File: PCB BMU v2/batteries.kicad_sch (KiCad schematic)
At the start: 19 parts, among them Q8 IRFZ44NPBF, U7 INA237

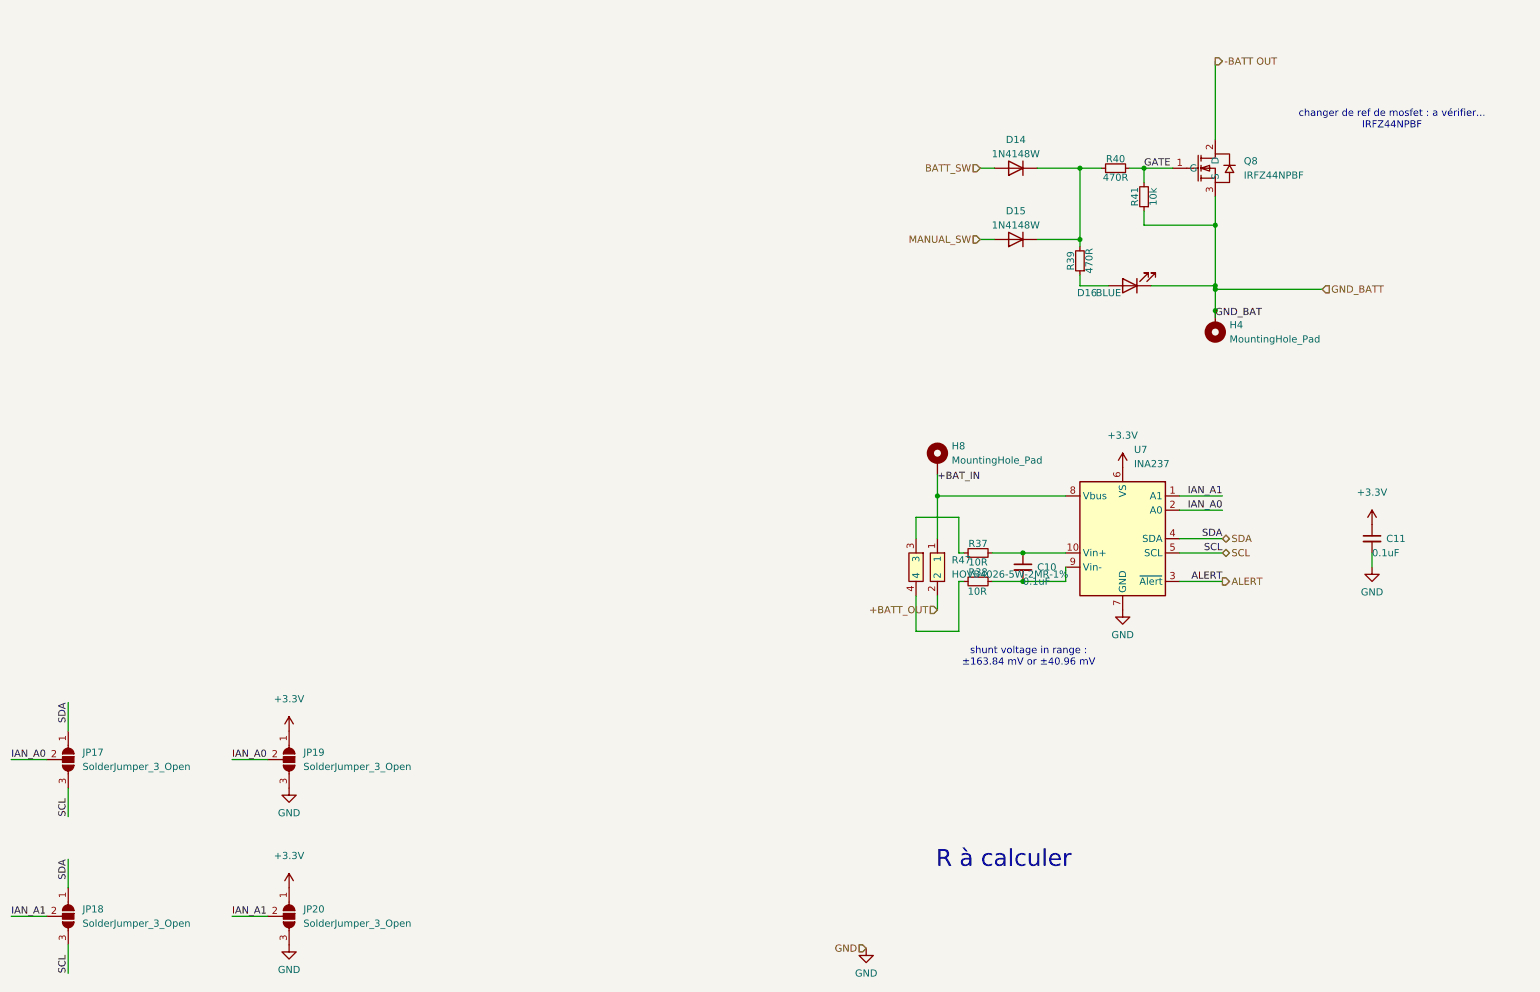
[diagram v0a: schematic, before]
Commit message: update code
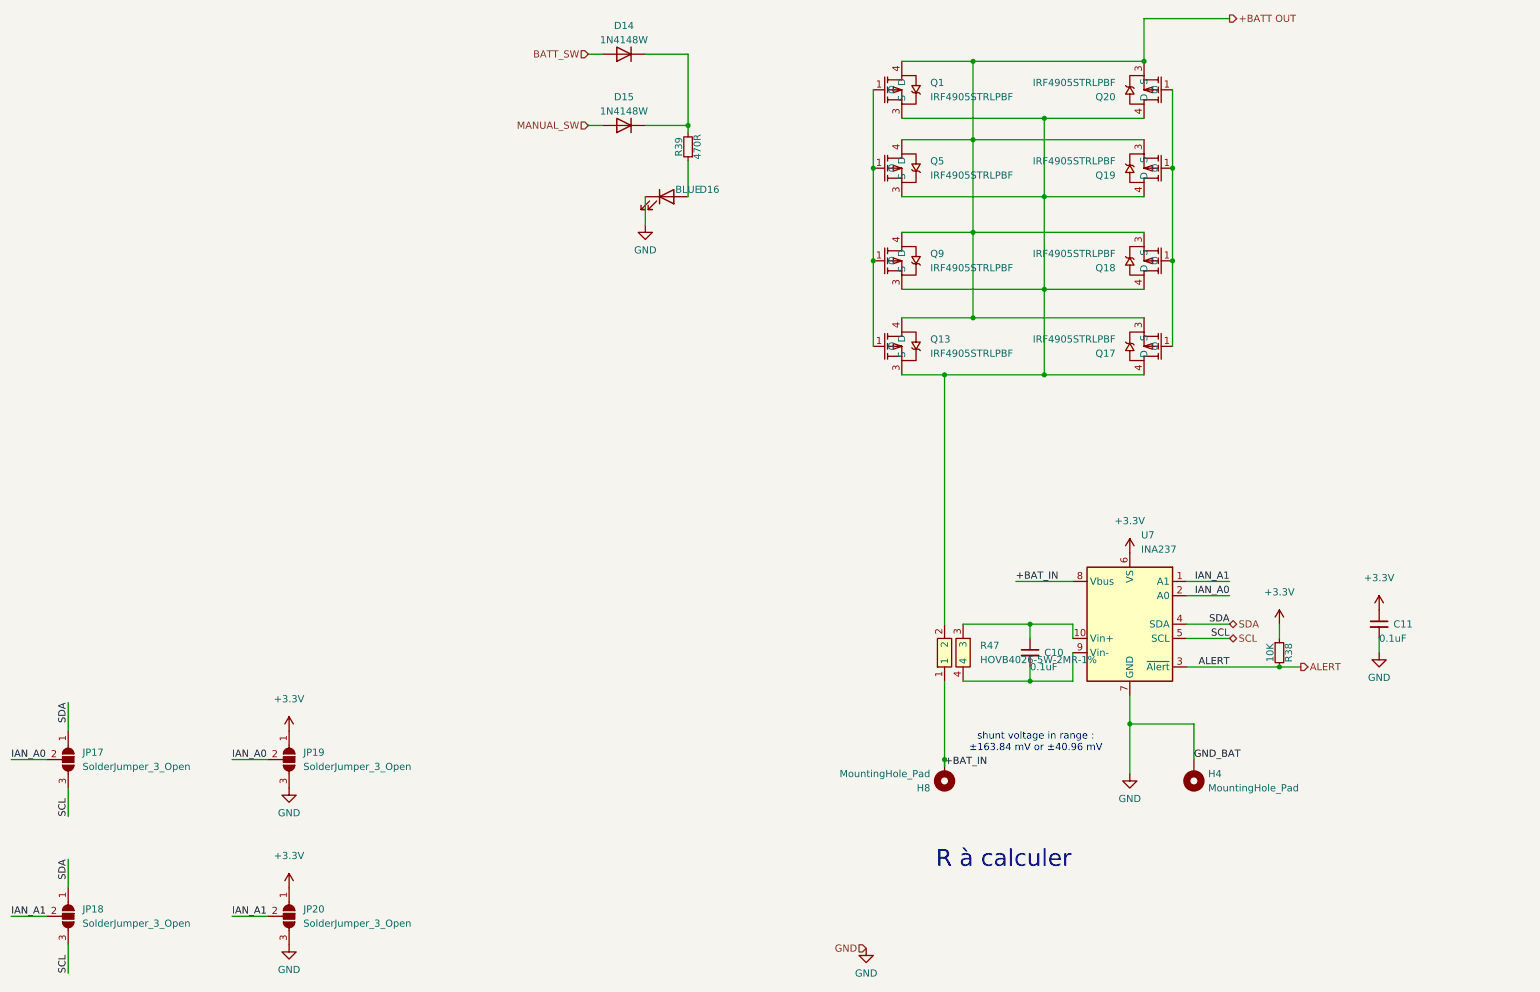
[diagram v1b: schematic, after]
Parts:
- removed Q8: IRFZ44NPBF, Package_TO_SOT_THT:TO-220-3_Horizontal_TabUp, symbol easyeda2kicad:IRFZ44NPBF
- removed R37: 10R, Resistor_SMD:R_0603_1608Metric, symbol Device:R_Small
- removed R40: 470R, Resistor_THT:R_Axial_DIN0204_L3.6mm_D1.6mm_P5.08mm_Horizontal, symbol Device:R_Small
- removed R41: 10k, Resistor_THT:R_Axial_DIN0204_L3.6mm_D1.6mm_P5.08mm_Horizontal, symbol Device:R_Small
- added Q1, Q13, Q17, Q18, Q19, Q20, Q5, Q9: IRF4905STRLPBF, easyeda2kicad:D2PAK_L9.1-W10.0-P2.54-LS15.3-TL, symbol easyeda2kicad:IRF4905STRLPBF
- C11: footprint Capacitor_SMD:C_0805_2012Metric -> Capacitor_SMD:C_0402_1005Metric; LCSC (none) -> C1525; LCSC Alt (none) -> C307331
- R38: value 10R -> 10K
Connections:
- net GND_BATT is gone; now on net GND: D16.1 (K), H4.1
- net +3.3V: now also R38.1
- net ALERT: now also R38.2
- net at R47.3: now also C10.1, U7.10 (Vin+)
- net at C10.2, U7.9 (Vin-): now also R47.4; no longer R38.1
- net +BATT_OUT: no longer names the net of R47.2
- net +BATT_OUT: now also Q1.3 (S), Q13.3 (S), Q17.4 (D), Q18.4 (D), Q19.4 (D), Q20.4 (D), Q5.3 (S), Q9.3 (S)
- new net: Q17.1 (G), Q18.1 (G), Q19.1 (G), Q20.1 (G)
- new net: Q1.1 (G), Q13.1 (G), Q5.1 (G), Q9.1 (G)
- new net +BATT OUT: Q1.4 (D), Q13.4 (D), Q17.3 (S), Q18.3 (S), Q19.3 (S), Q20.3 (S), Q5.4 (D), Q9.4 (D)
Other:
- note removed: "changer de ref de mosfet : a vérifier... IRFZ44NPBF"
- moved on the sheet: C10, C11, D14, D15, R39, R47, U7
